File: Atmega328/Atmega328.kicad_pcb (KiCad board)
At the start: 2 copper layers, 48.3 x 66 mm, 30 parts, among them J1 Conn_01x02, J2 Conn_02x03_Odd_Even, J3 Conn_01x14, SW1 SW_Push, U1 LM358, U2 LM358, U3 LM78M05_TO252, U4 ATmega328P-PU, U5 DHT11, Y1 12MHz

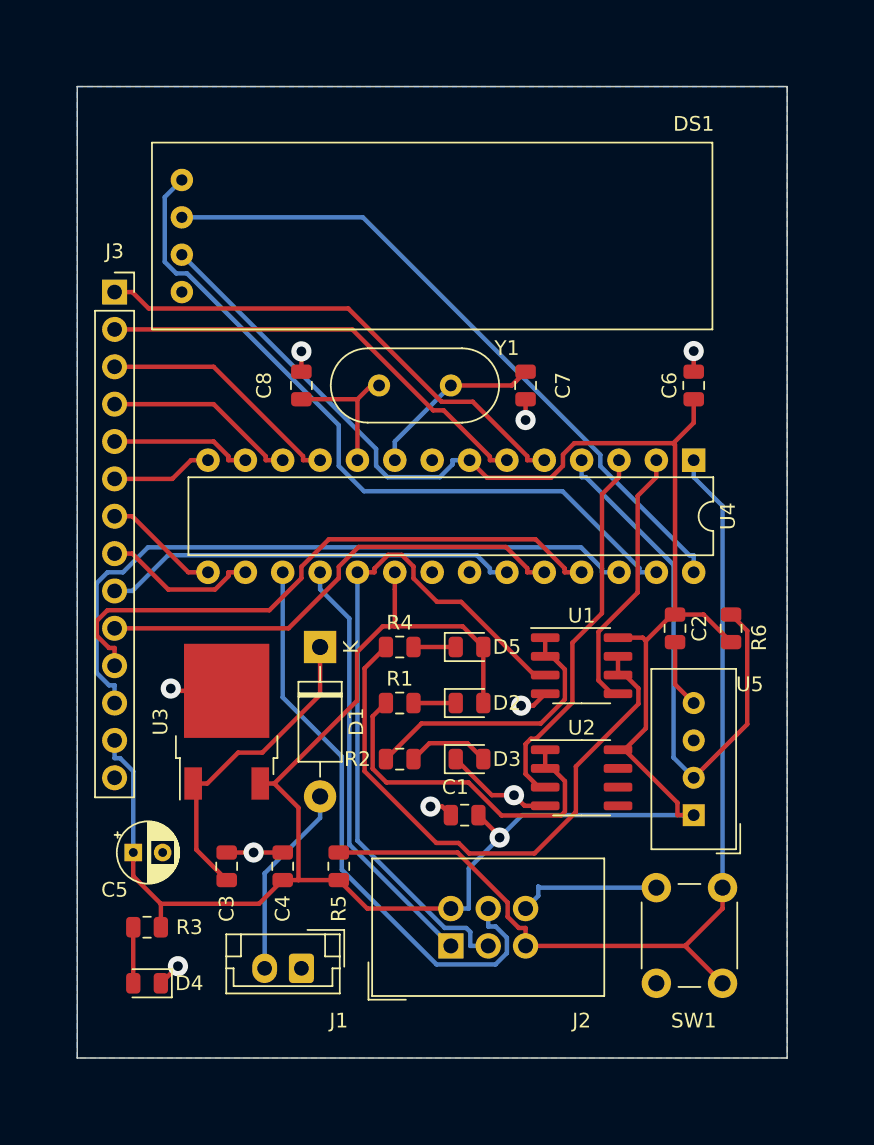
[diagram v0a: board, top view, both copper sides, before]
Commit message: PCB Cleanup and Ready
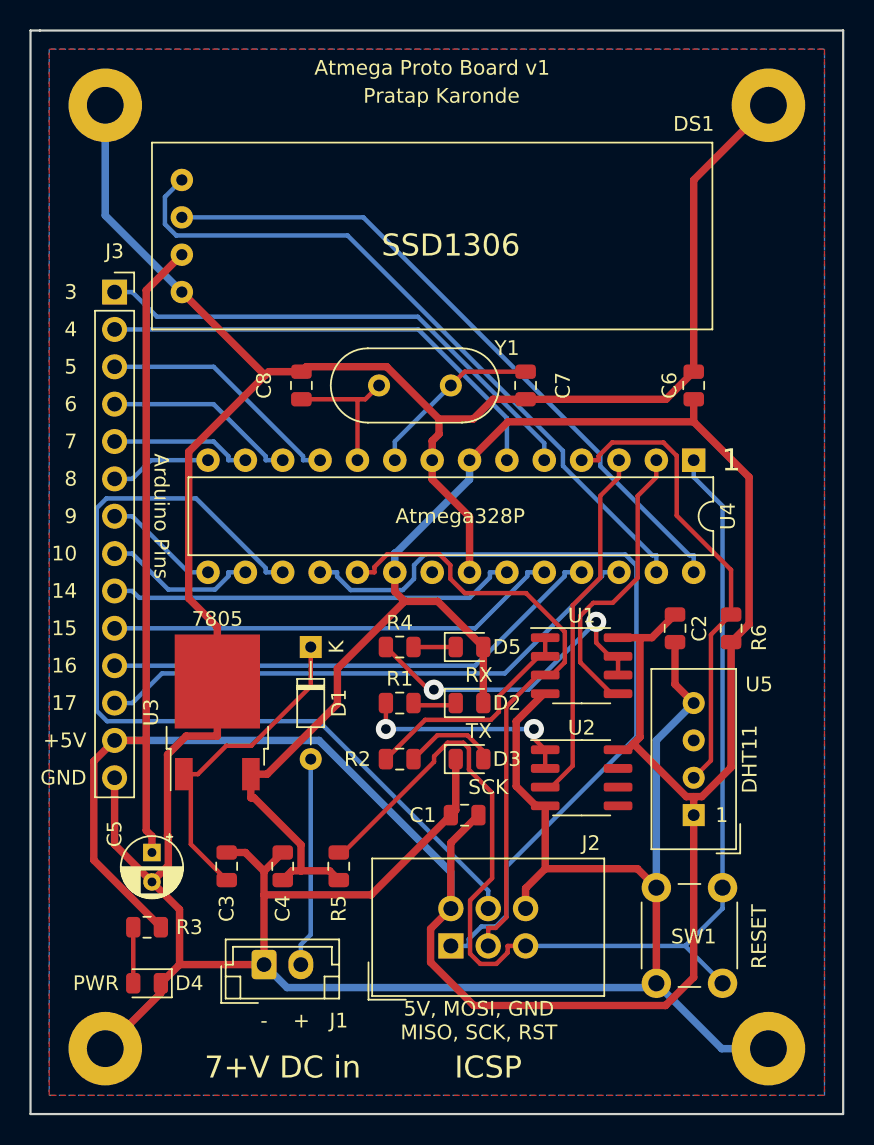
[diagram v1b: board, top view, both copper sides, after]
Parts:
- added M1: MountingHole_2.5mm_Pad, MountingHole:MountingHole_2.5mm_Pad, F.Cu at (84.5, 26.7)
- added M2: MountingHole_2.5mm_Pad, MountingHole:MountingHole_2.5mm_Pad, F.Cu at (129.5, 26.7)
- added M3: MountingHole_2.5mm_Pad, MountingHole:MountingHole_2.5mm_Pad, F.Cu at (129.5, 90.8)
- added M4: MountingHole_2.5mm_Pad, MountingHole:MountingHole_2.5mm_Pad, F.Cu at (84.5, 90.8)
- D1: footprint Diode_THT:D_DO-41_SOD81_P10.16mm_Horizontal -> Diode_THT:D_DO-34_SOD68_P7.62mm_Horizontal
- moved J1 2.55 mm to (95.2, 85.1), turned to 0 degrees
- moved C5 1.27 mm to (87.6, 77.5), turned to 270 degrees
- moved U3 0.90 mm to (92.1, 67.9)
- moved D1 0.64 mm to (98.4, 63.5)
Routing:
- net GND: track 39.1 -> 272.6 mm, vias 9 -> 0
- net +5V: track 178.1 -> 248.8 mm, vias 1 -> 0
- net /MISO: track 29.1 -> 56.4 mm
- net /MOSI: track 39.9 -> 61.8 mm
- net Net-(R4-Pad1): track 40.1 -> 22.0 mm, vias 0 -> 2
- net /RESET: track 65.9 -> 81.7 mm
- net Net-(R1-Pad1): track 24.4 -> 14.8 mm, vias 0 -> 2
- net /ARD_17: track 46.3 -> 38.1 mm
- net /ARD_16: track 40.6 -> 34.5 mm
- net /SCK: track 47.9 -> 41.9 mm
- net /ARD_2: track 38.0 -> 32.0 mm
- net Net-(R2-Pad1): track 18.9 -> 15.6 mm
- net /SDA: track 50.0 -> 48.0 mm
- net /ARD_15: track 32.8 -> 30.9 mm
- net /RXLED: track 18.3 -> 20.1 mm
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- added copper zone on F.Cu, net GND
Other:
- board size 48.3 x 66 mm -> 55.2 x 73.7 mm
- board text added: "+"
- board text added: "+5V"
- board text added: "-"
- board text added: "1"
- board text added: "10"
- board text added: "14"
- board text added: "15"
- board text added: "16"
- board text added: "17"
- board text added: "3"
- board text added: "4"
- board text added: "5"
- board text added: "5V, MOSI, GND MISO, SCK, RST"
- board text added: "6"
- board text added: "7"
- board text added: "7+V DC in"
- board text added: "7805"
- board text added: "8"
- board text added: "9"
- board text added: "Arduino Pins"
- board text added: "Atmega Proto Board v1"
- board text added: "Atmega328P"
- board text added: "DHT11"
- board text added: "GND"
- board text added: "ICSP"
- board text added: "PWR"
- board text added: "Pratap Karonde"
- board text added: "RESET"
- board text added: "RX"
- board text added: "SCK"
- board text added: "SSD1306"
- board text added: "TX"
